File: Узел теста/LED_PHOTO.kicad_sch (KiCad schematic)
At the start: 10 parts

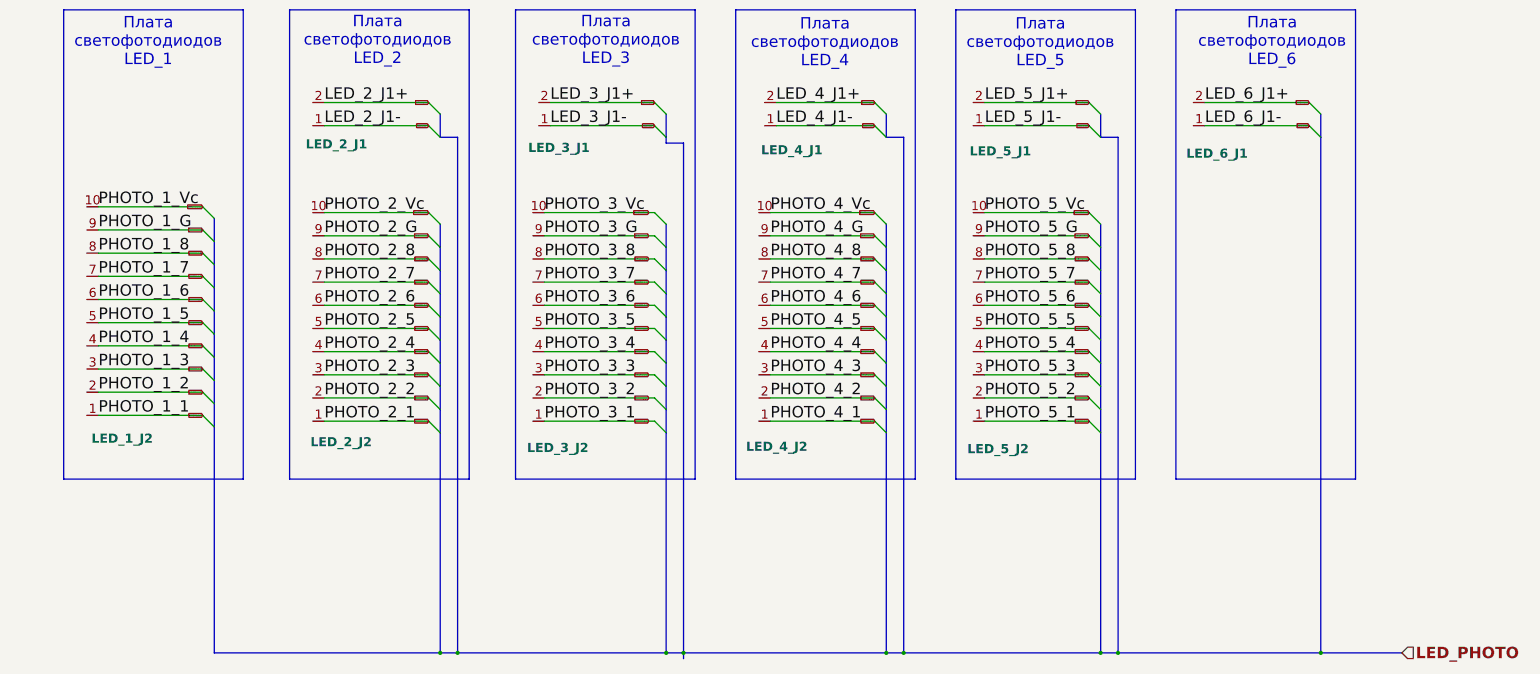
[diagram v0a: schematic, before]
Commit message: update schemas
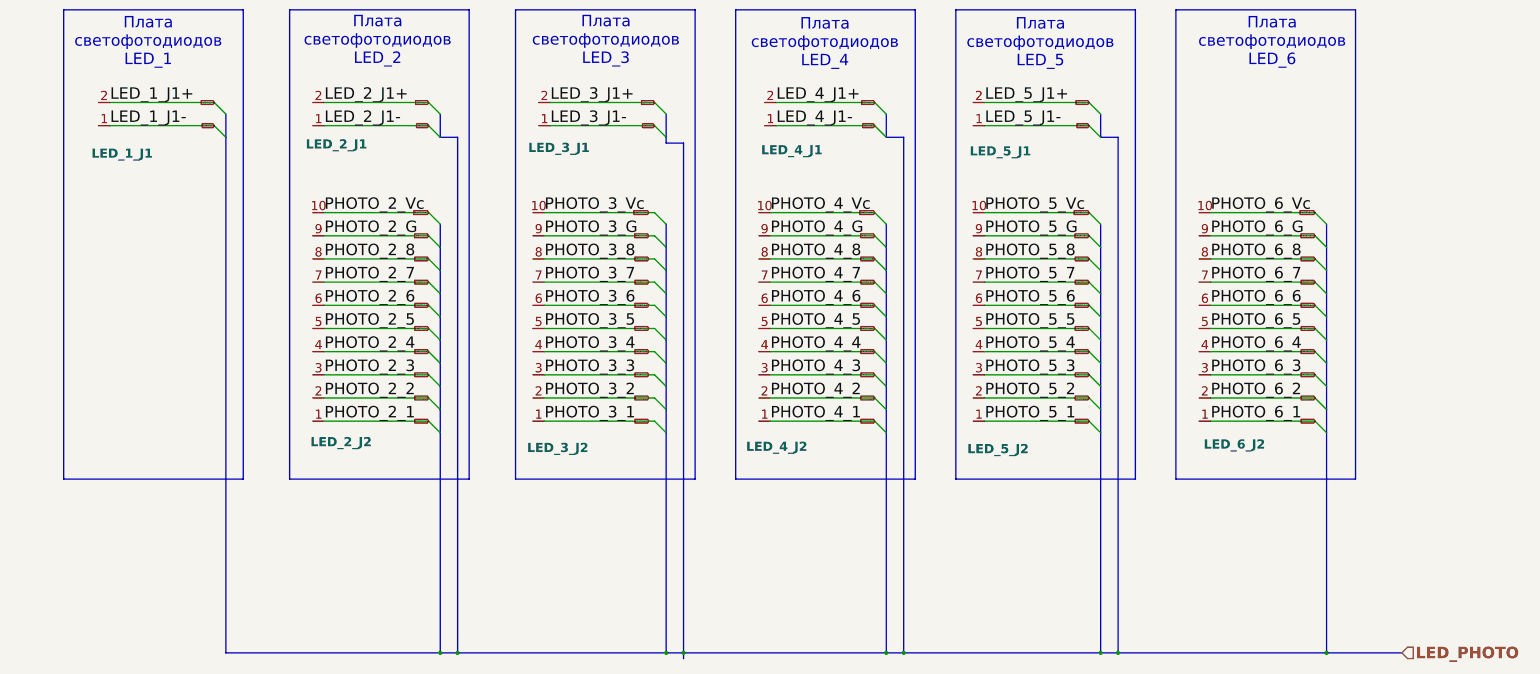
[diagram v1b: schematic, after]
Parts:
- renumbered LED_6_J1 to LED_1_J1, LED_1_J2 to LED_6_J2
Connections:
- net LED_6_J1+ renamed LED_1_J1+
- net LED_6_J1- renamed LED_1_J1-
- net PHOTO_1_1 renamed PHOTO_6_1
- net PHOTO_1_2 renamed PHOTO_6_2
- net PHOTO_1_3 renamed PHOTO_6_3
- net PHOTO_1_4 renamed PHOTO_6_4
- net PHOTO_1_5 renamed PHOTO_6_5
- net PHOTO_1_6 renamed PHOTO_6_6
- net PHOTO_1_7 renamed PHOTO_6_7
- net PHOTO_1_8 renamed PHOTO_6_8
- net PHOTO_1_G renamed PHOTO_6_G
- net PHOTO_1_Vc renamed PHOTO_6_Vc
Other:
- moved on the sheet: LED_1_J1, LED_6_J2
